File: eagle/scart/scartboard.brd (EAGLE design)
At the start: 100 x 80 mm, 42 parts, among them Q1 BC548-TO92-E1-REV, Q2 BC548-TO92-E1-REV, Q3 BC548-TO92-E1-REV, Q4 BC548-TO92-E1-REV, T1 BSS138, T3 BSS138, X1 SCART-F

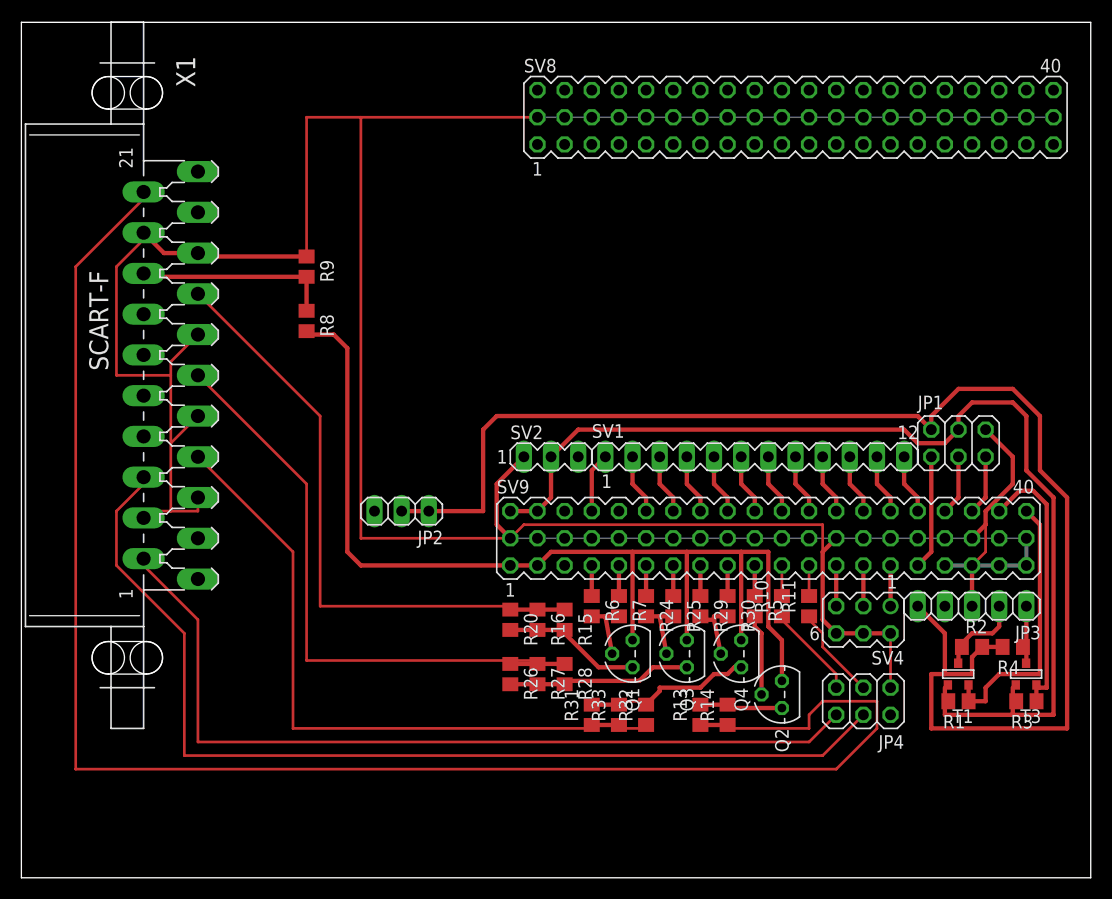
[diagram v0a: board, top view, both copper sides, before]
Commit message: WIP
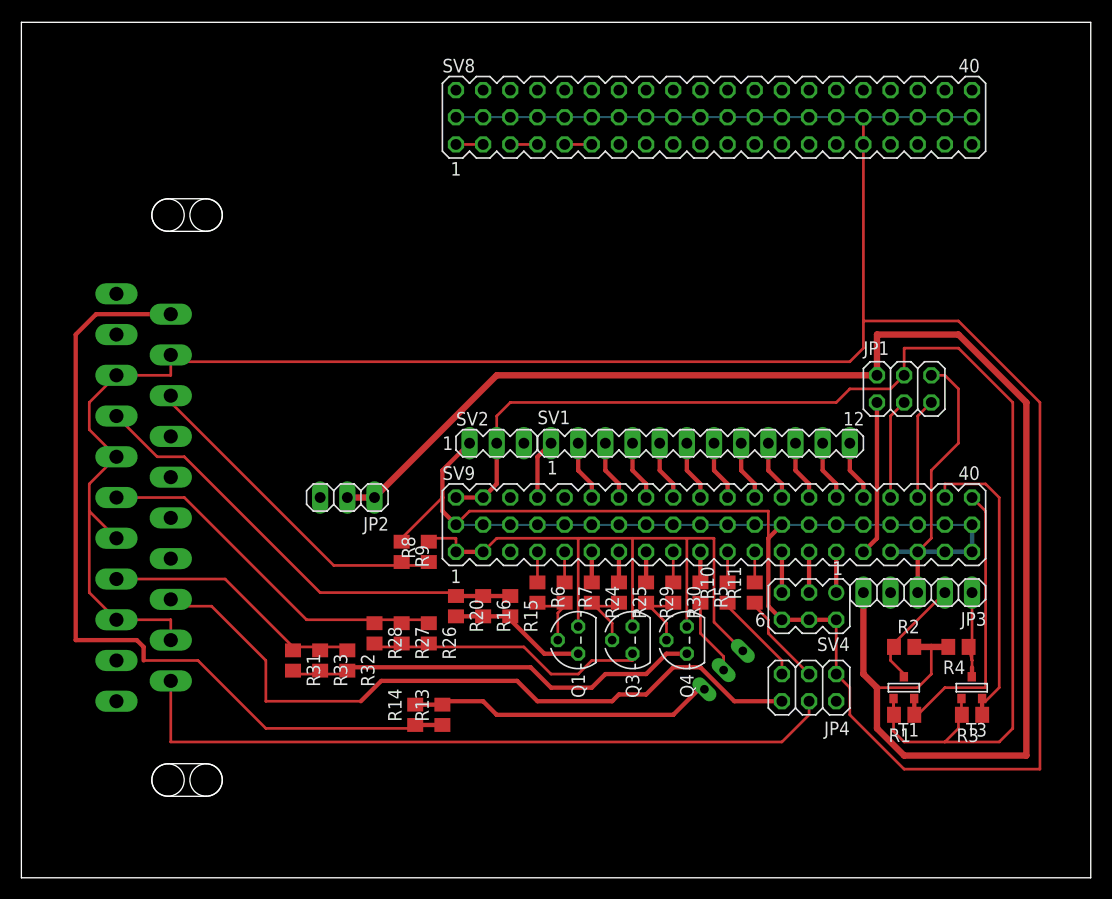
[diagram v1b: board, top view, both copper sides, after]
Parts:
- Q2: value BC548-TO92-E1-REV -> BC548; device bc548:TO92-E1-REV -> transistor-npn:TO92-EBC
- R8: value 1000 -> 75
- R9: value 1000 -> 750
- moved R14 29.2 mm to (36.8, 15.2)
- moved R31 28.4 mm to (25.4, 20.3), turned to 270 degrees
- moved R32 28.4 mm to (30.5, 20.3), turned to 270 degrees
- moved R33 28.4 mm to (27.9, 20.3), turned to 270 degrees
- moved R9 28.1 mm to (35.6, 30.5)
- moved R8 24.4 mm to (38.1, 30.5), turned to 90 degrees
- moved R13 24.1 mm to (39.4, 15.2)
- moved R28 18.2 mm to (33.0, 22.9)
- moved R27 13.3 mm to (35.6, 22.9)
- moved X1 11.7 mm to (14.0, 35.6), flipped to the bottom
- moved R26 8.52 mm to (38.1, 22.9)
- moved SV8 7.62 mm to (64.8, 71.1)
- moved JP1 7.18 mm to (82.5, 45.7)
- moved Q2 7.10 mm to (64.8, 20.3), flipped to the bottom, turned to 315 degrees
- moved R2 6.35 mm to (82.5, 21.6)
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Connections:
- new net VCC_CORE: SV8.1, SV8.3
- net ALEFT: now also JP4.6; no longer JP4.4
- net ARIGHT: now also JP4.4; no longer JP4.6
- net N$1: now also Q2.E; no longer Q2.3
- net N$3: now also Q2.B; no longer Q2.2
- net VCC_B0: now also SV8.7
- net VCC_B1: now also SV8.11
- net VCC_B3: now also Q2.C; no longer Q2.1
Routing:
- net COMP: track 154.3 -> 77.0 mm
- net GND: track 244.4 -> 311.5 mm
- net BLUE: track 63.1 -> 25.2 mm
- net VCC_B3: track 101.3 -> 65.2 mm
- net ALEFT: track 94.8 -> 67.9 mm
- net N$12: track 16.2 -> 40.0 mm
- net GREEN: track 58.2 -> 34.9 mm
- net N$1: track 8.20 -> 28.7 mm
- net VCC_B2: track 102.9 -> 117.1 mm
- net D_FASTBLANKING: track 18.6 -> 32.4 mm
- net RED: track 57.4 -> 44.3 mm
- net ARIGHT: track 80.6 -> 67.7 mm
- net VCC_5V: track 135.8 -> 147.3 mm
- net N$10: track 17.6 -> 27.3 mm
- net CASMOTOR: track 5.61 -> 9.42 mm
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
